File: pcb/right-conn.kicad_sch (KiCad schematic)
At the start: 19 parts, among them J5 USB_C_Plug, J6 USB_C_Receptacle

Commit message: Added MPNs and footprints for I think everything.
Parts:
- J5: footprint (none) -> Connector_USB:USB_C_Receptacle_GCT_USB4085; MPN (none) -> USB4085-GF-A
- J6: footprint (none) -> Connector_USB:USB_C_Receptacle_Amphenol_12401548E4-2A; MPN (none) -> 12401548E4#2A
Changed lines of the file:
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@@
 			)
 		)
-		(property "Footprint" ""
+		(property "Footprint" "Connector_USB:USB_C_Receptacle_Amphenol_12401548E4-2A"
 			(at 99.06 181.61 0)
 			(effects
@@
 		)
 		(property "Description" "USB Full-Featured Type-C Receptacle connector"
+			(at 95.25 181.61 0)
+			(effects
+				(font
+					(size 1.27 1.27)
+				)
+				(hide yes)
+			)
+		)
+		(property "MPN" "12401548E4#2A "
 			(at 95.25 181.61 0)
 			(effects
@@
 			)
 		)
-		(property "Footprint" ""
+		(property "Footprint" "Connector_USB:USB_C_Receptacle_GCT_USB4085"
 			(at 99.06 57.15 0)
 			(effects
@@
 			(at 95.25 57.15 0)
 			(effects
+				(font
+					(size 1.27 1.27)
+				)
+				(hide yes)
+			)
+		)
+		(property "MPN" "USB4085-GF-A "
+			(at 95.25 57.15 0)
+			(effects

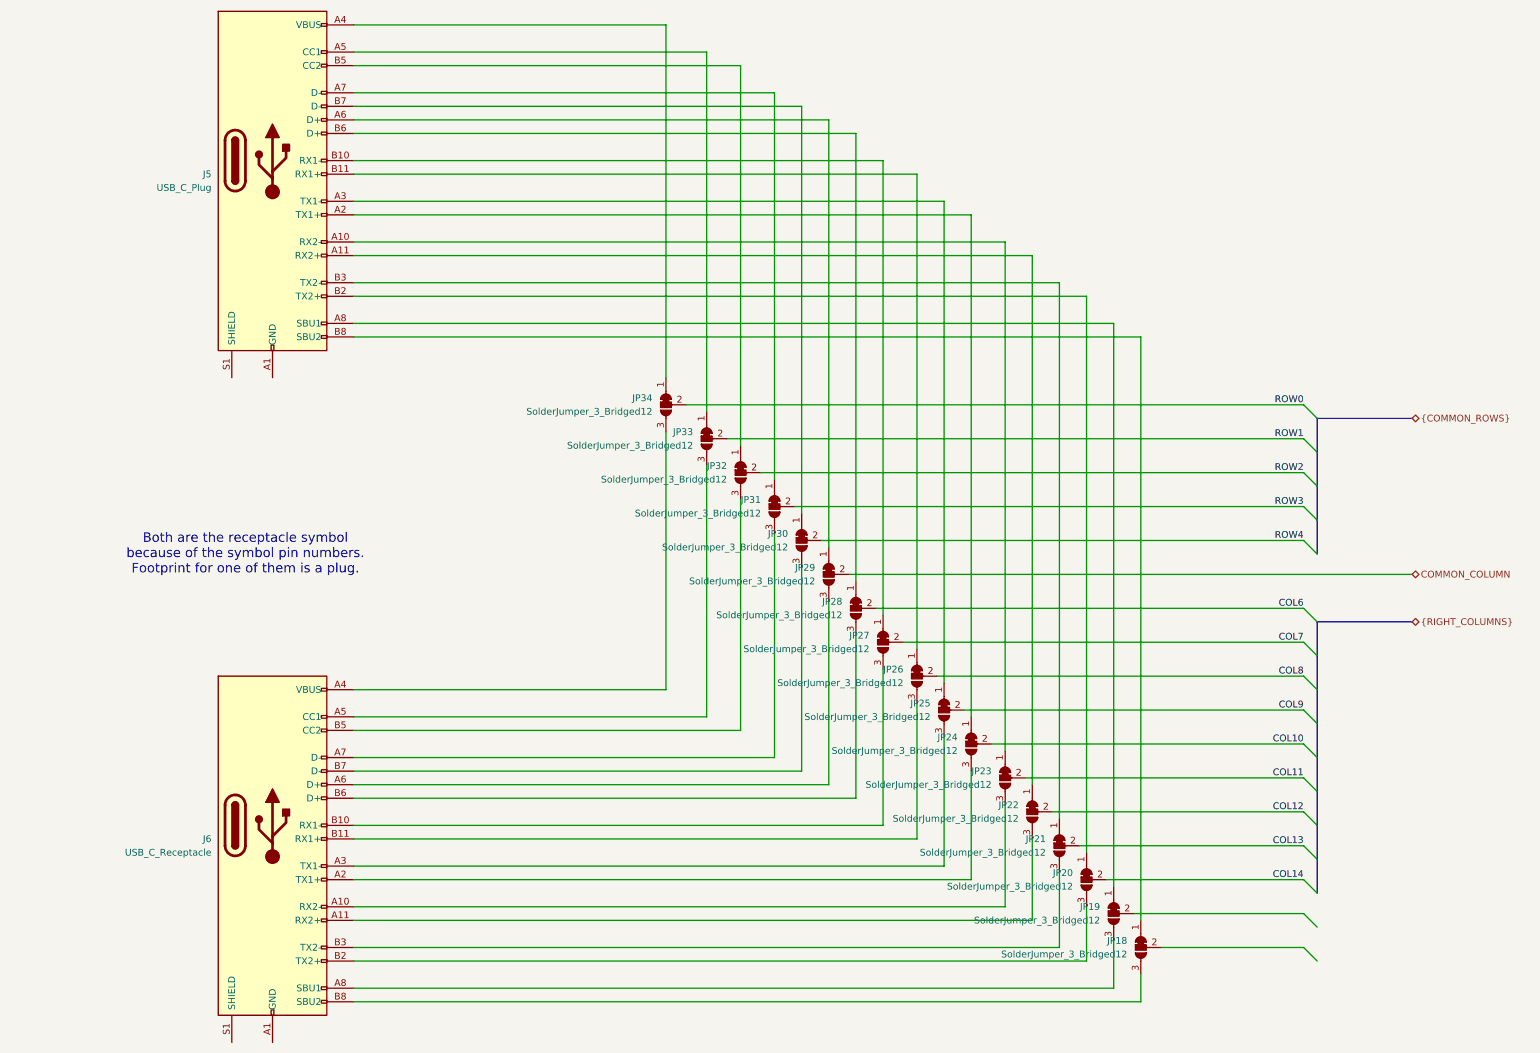
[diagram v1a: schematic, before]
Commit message: Continuing...no one will read this but me.
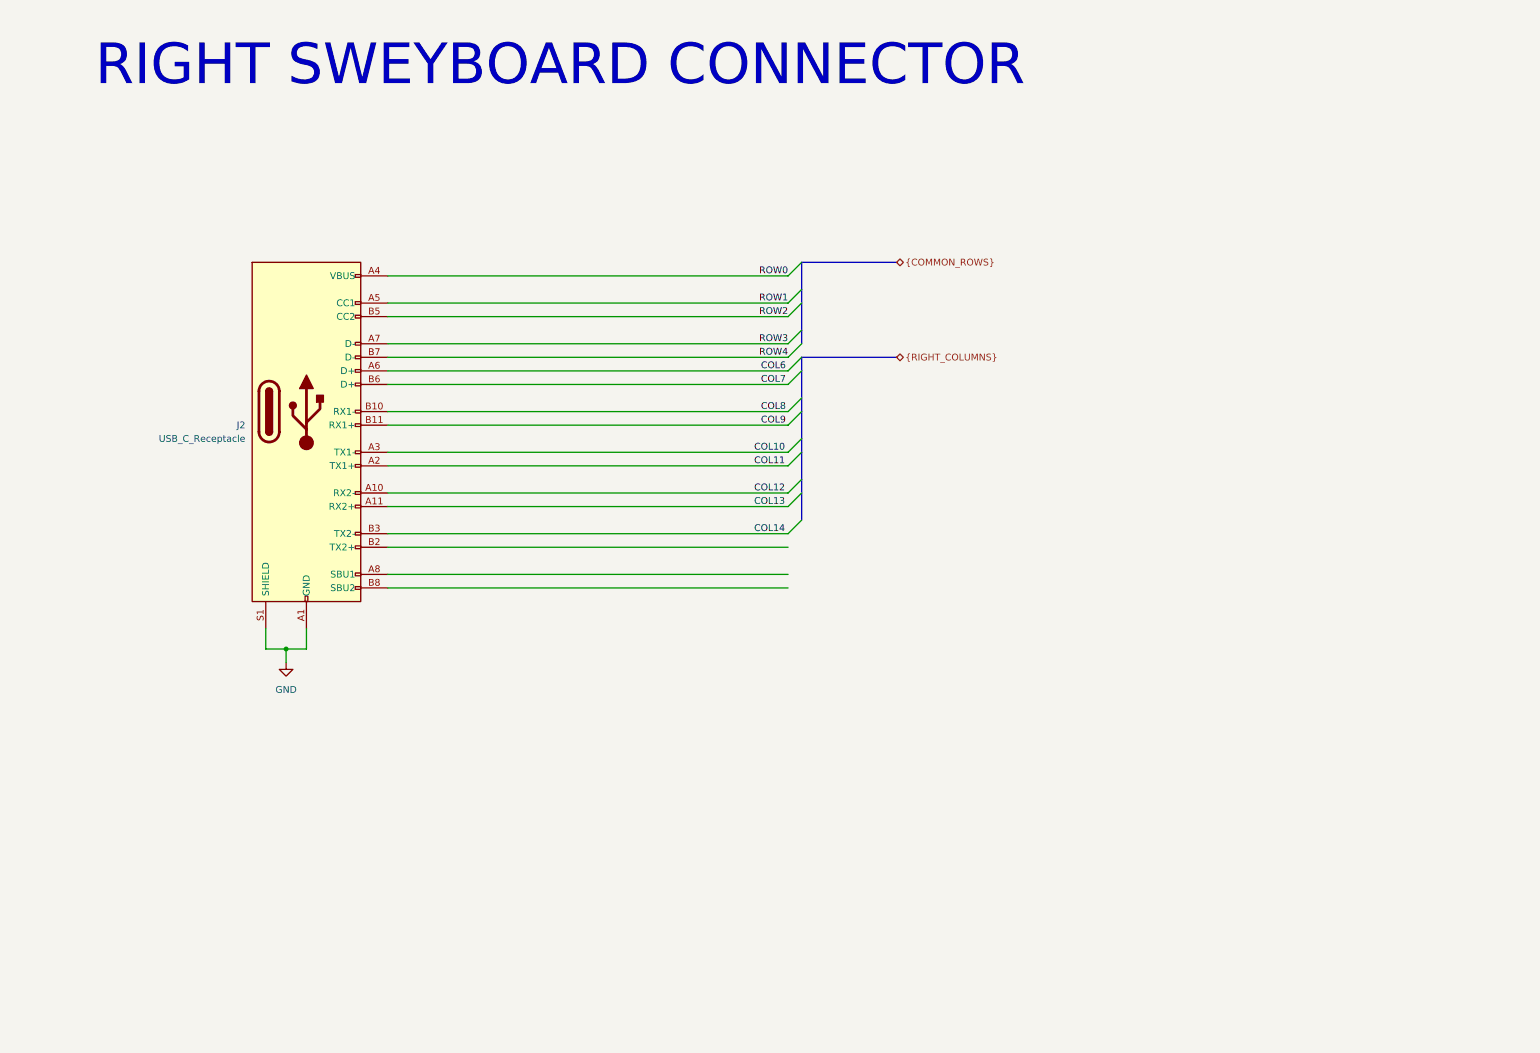
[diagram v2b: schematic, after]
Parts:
- removed J5: USB_C_Plug, Connector_USB:USB_C_Receptacle_GCT_USB4085, symbol Connector:USB_C_Receptacle
- removed J6: USB_C_Receptacle, Connector_USB:USB_C_Receptacle_Amphenol_12401548E4-2A, symbol Connector:USB_C_Receptacle
- removed JP18, JP19, JP20, JP21, JP22, JP23, JP24, JP25, JP26, JP27, JP28, JP29, JP30, JP31, JP32, JP33, JP34: SolderJumper_3_Bridged12, Jumper:SolderJumper-3_P1.3mm_Bridged12_Pad1.0x1.5mm, symbol Jumper:SolderJumper_3_Bridged12
- added J2: USB_C_Receptacle, Connector_USB:USB_C_Receptacle_Amphenol_12401548E4-2A, symbol Connector:USB_C_Receptacle
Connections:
- net COL10: now also J2.A3 (TX1-)
- net COL11: now also J2.A2 (TX1+)
- net COL12: now also J2.A10 (RX2-)
- net COL13: now also J2.A11 (RX2+)
- net COL14: now also J2.B3 (TX2-)
- net COL6: now also J2.A6 (D+)
- net COL7: now also J2.B6 (D+)
- net COL8: now also J2.B10 (RX1-)
- net COL9: now also J2.B11 (RX1+)
- net ROW0: now also J2.A4 (VBUS), J2.A9 (VBUS), J2.B4 (VBUS), J2.B9 (VBUS)
- net ROW1: now also J2.A5 (CC1)
- net ROW2: now also J2.B5 (CC2)
- net ROW3: now also J2.A7 (D-)
- net ROW4: now also J2.B7 (D-)
- new net GND: J2.A1 (GND), J2.A12 (GND), J2.B1 (GND), J2.B12 (GND), J2.S1 (SHIELD)
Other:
- note added: "RIGHT SWEYBOARD CONNECTOR"
- note removed: "Both are the receptacle symbol because of the symbol pin numbers. Footprint for one of them is a plug."
